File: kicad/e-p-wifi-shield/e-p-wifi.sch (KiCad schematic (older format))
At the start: 31 parts, among them J1 T1, J2 Masse, J3 T2, J4 Conn_02x14_MKR1010, SW1 Conrad 711771, SW2 StSp, SW3 Sleep

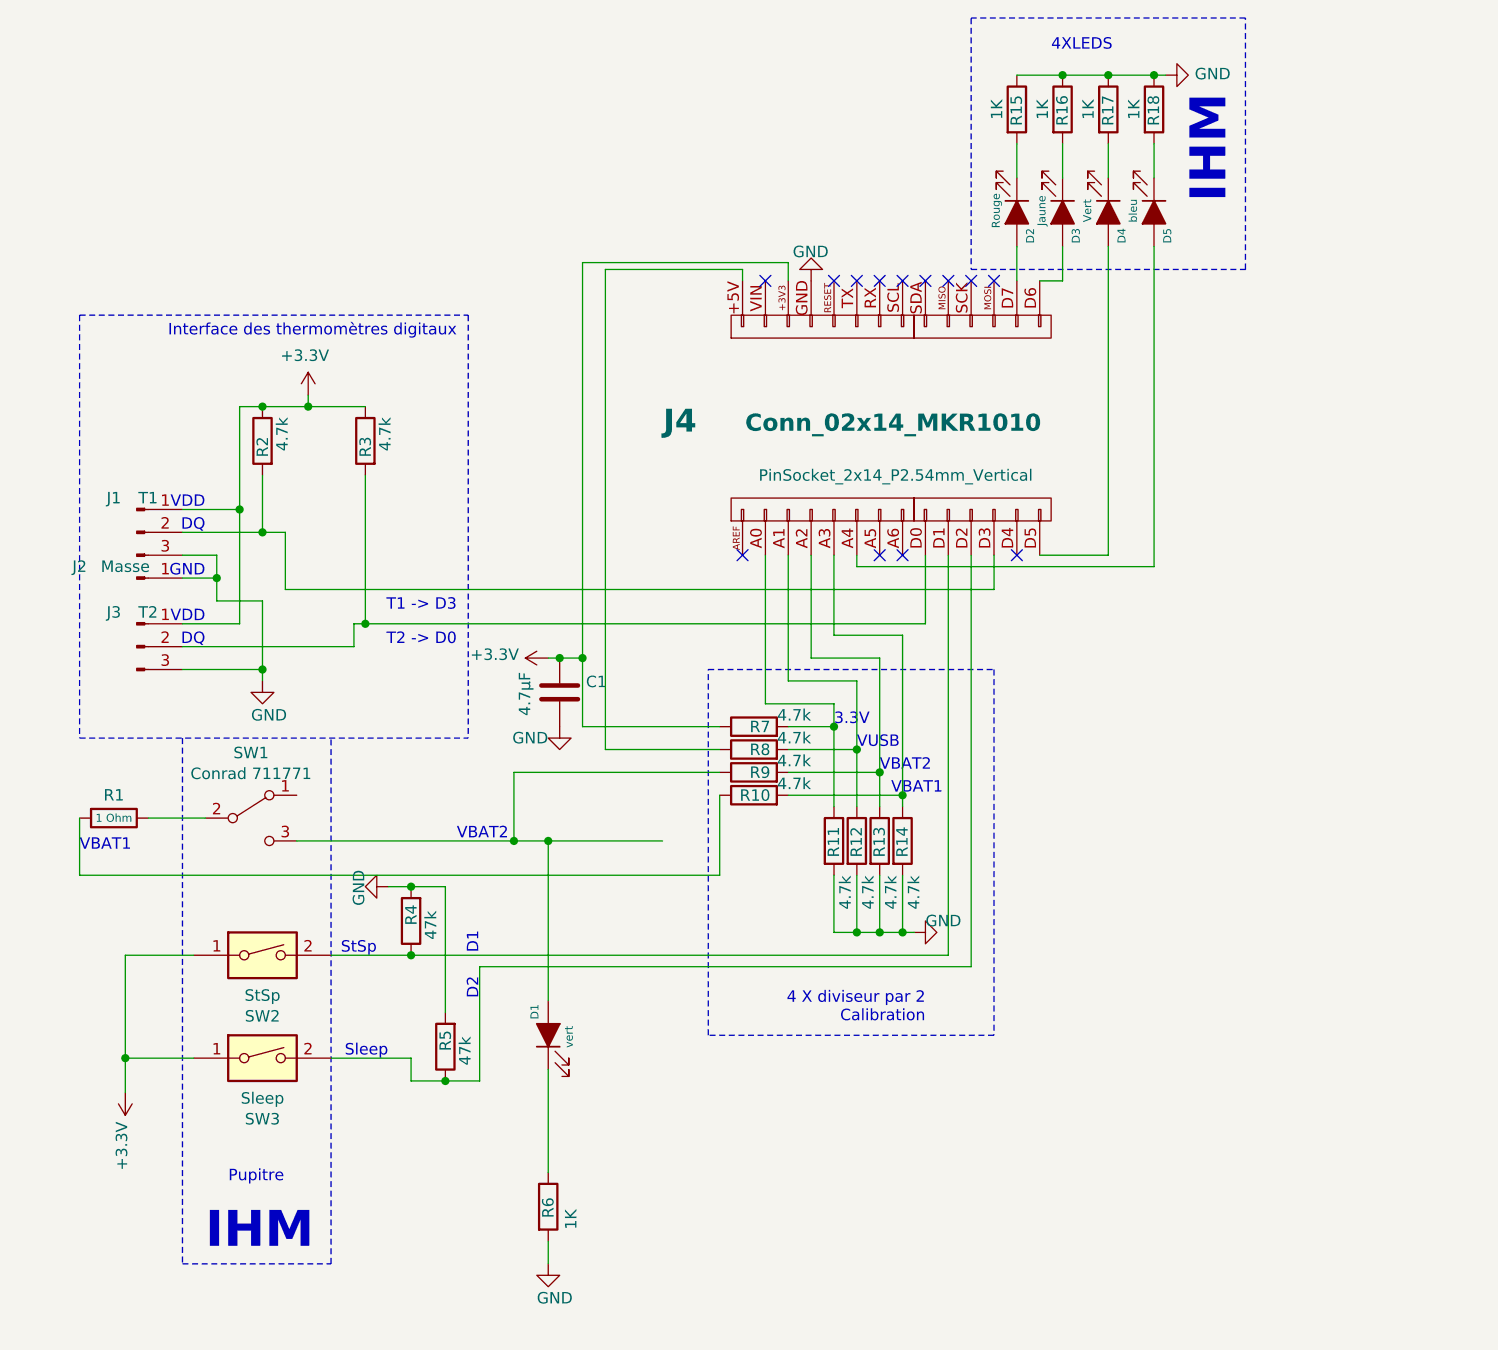
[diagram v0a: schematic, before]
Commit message: Maj du 07 novembre 2019
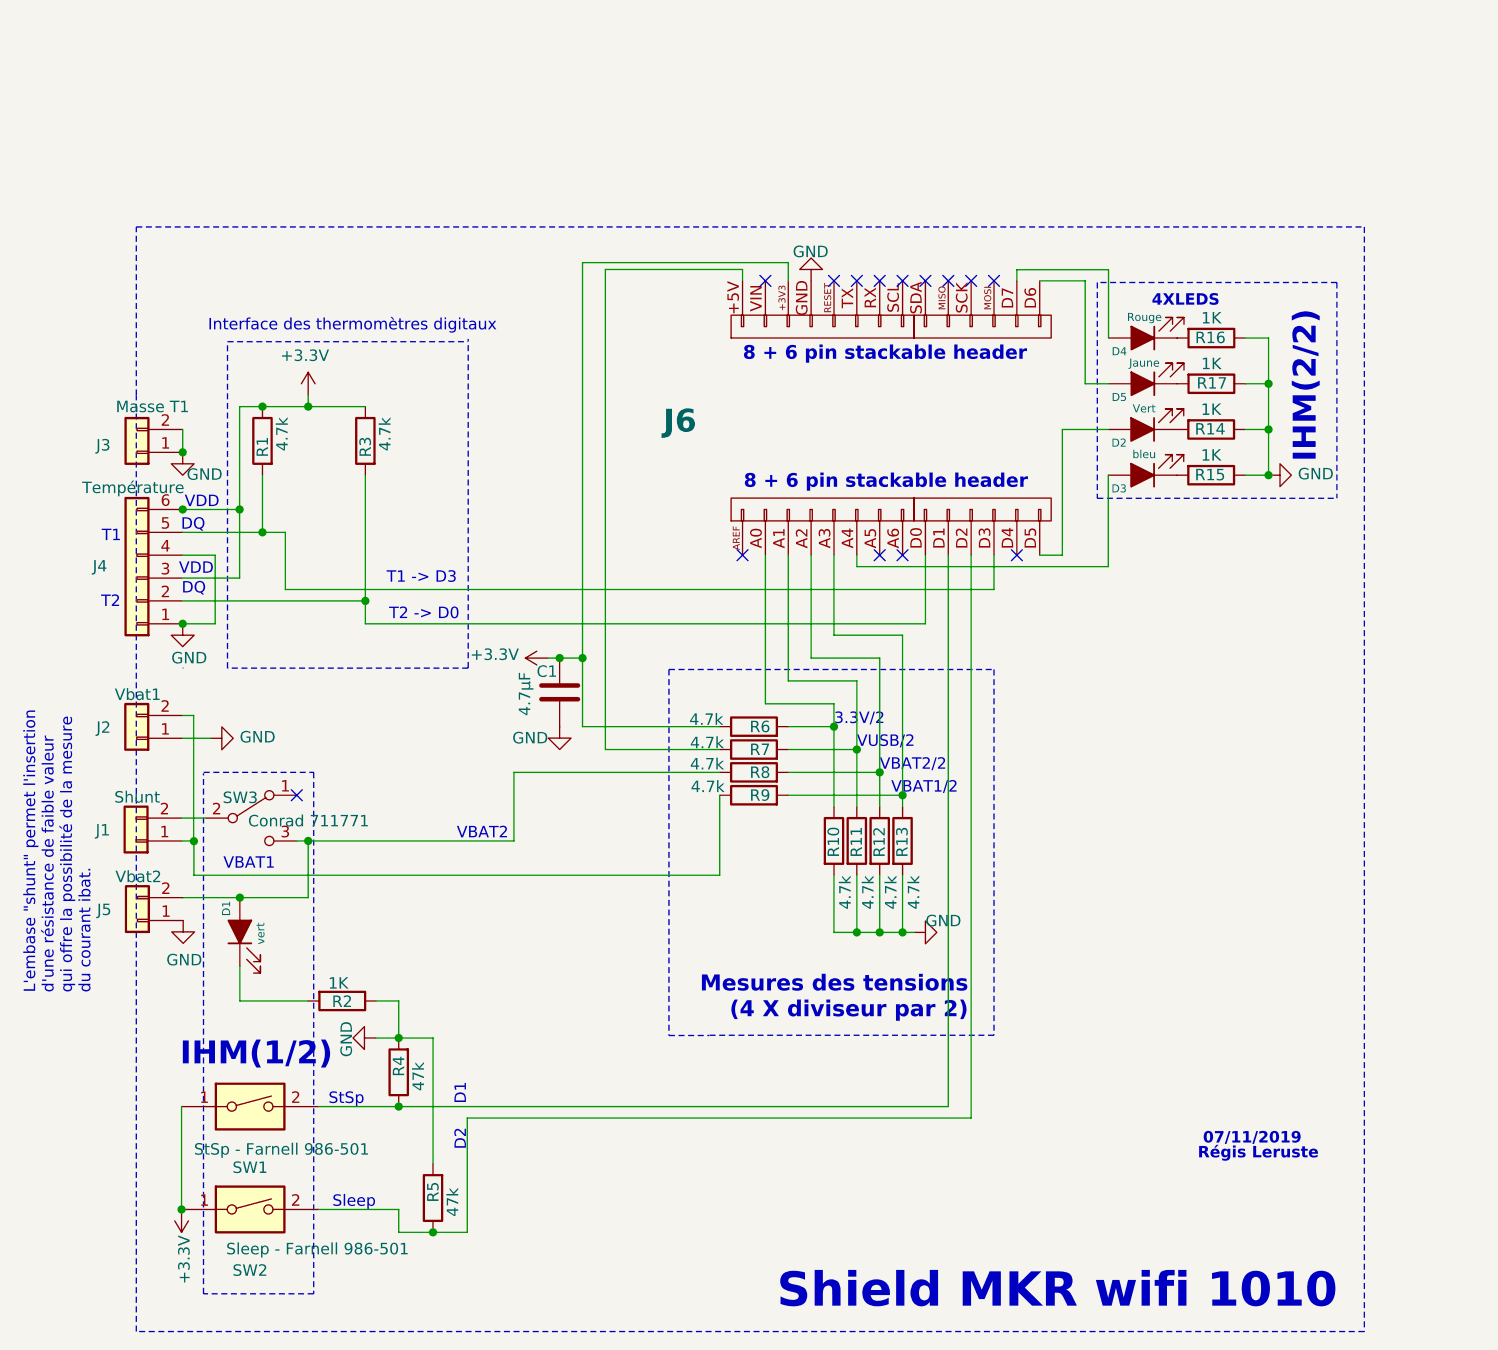
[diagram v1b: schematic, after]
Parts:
- removed J1: T1, symbol Connector:Conn_01x03_Male
- removed J2: Masse, symbol Connector:Conn_01x01_Male
- removed J3: T2, symbol Connector:Conn_01x03_Male
- removed R1: 1 Ohm, Resistor_THT:R_Axial_DIN0207_L6.3mm_D2.5mm_P7.62mm_Horizontal, symbol Device:R
- added J1: Shunt, Connector_PinHeader_2.54mm:PinHeader_1x02_P2.54mm_Vertical, symbol Connector_Generic:Conn_01x02
- added J2: Vbat1, Connector_PinHeader_2.54mm:PinHeader_1x02_P2.54mm_Vertical, symbol Connector_Generic:Conn_01x02
- added J3: Masse T1, Connector_PinHeader_2.54mm:PinHeader_1x02_P2.54mm_Vertical, symbol Connector_Generic:Conn_01x02
- added J4: Température, Connector_PinHeader_1.00mm:PinHeader_1x06_P1.00mm_Vertical, symbol Connector_Generic:Conn_01x06
- added J5: Vbat2, Connector_PinHeader_2.54mm:PinHeader_1x02_P2.54mm_Vertical, symbol Connector_Generic:Conn_01x02
- J6: renamed from J4; footprint PinSocket_2x14_P2.54mm_Vertical -> MKR1010:PinSocket_2x14_MKR1010
- SW1: renamed from SW2; value StSp -> StSp - Farnell 986-501; footprint (none) -> MKR1010:jumper-switch
- SW2: renamed from SW3; value Sleep -> Sleep - Farnell 986-501; footprint (none) -> MKR1010:jumper-switch
- SW3: renamed from SW1; footprint (none) -> MKR1010:switch
- renumbered D4 to D2, D5 to D3, D2 to D4, D3 to D5, R2 to R1, R11 to R10, R12 to R11, R13 to R12, R14 to R13, R17 to R14, R18 to R15, R15 to R16, R16 to R17, R6 to R2, R7 to R6, R8 to R7, R9 to R8, R10 to R9
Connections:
- net +3V3: now also J4.3 (Pin_3), J4.6 (Pin_6)
- net GND: now also R2.1, J2.1 (Pin_1), J3.1 (Pin_1), J3.2 (Pin_2), J4.1 (Pin_1), J4.4 (Pin_4), J5.1 (Pin_1); no longer R2.2
- net at D1.2 (A), R8.1, SW3.3 (C): now also J5.2 (Pin_2)
- net at R9.1: now also J1.1 (Pin_1), J2.2 (Pin_2)
- net at J6.D0 (Pin_9), R3.2: now also J4.2 (Pin_2)
- net at J6.D3 (Pin_12), R1.2: now also J4.5 (Pin_5)
- net at SW3.2 (B): now also J1.2 (Pin_2)
- net at D1.1 (K): now also R2.2; no longer R2.1
- no-connect marks 13 -> 14
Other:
- note added: "07/11/2019"
- note added: "3.3V/2"
- note added: "8 + 6 pin stackable header"
- note added: "IHM(1/2)"
- note added: "IHM(2/2)"
- note added: "L'embase "shunt" permet l'insertion\nd'une résistance de faible valeur\nqui offre la possibilité de la mesure\ndu courant ibat."
- note added: "Mesures des tensions\n(4 X diviseur par 2)"
- note added: "Régis Leruste"
- note added: "Shield MKR wifi 1010"
- note added: "T1"
- note added: "T2"
- note added: "VBAT1/2"
- note added: "VBAT2/2"
- note added: "VUSB/2"
- note removed: "3.3V"
- note removed: "4 X diviseur par 2\nCalibration"
- note removed: "GND"
- note removed: "IHM"
- note removed: "Pupitre"
- note removed: "VUSB"
- moved on the sheet: D1, D2, D3, D4, D5, R14, R15, R16, R17, R2, R4, R5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
